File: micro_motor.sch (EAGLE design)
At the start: 56 parts

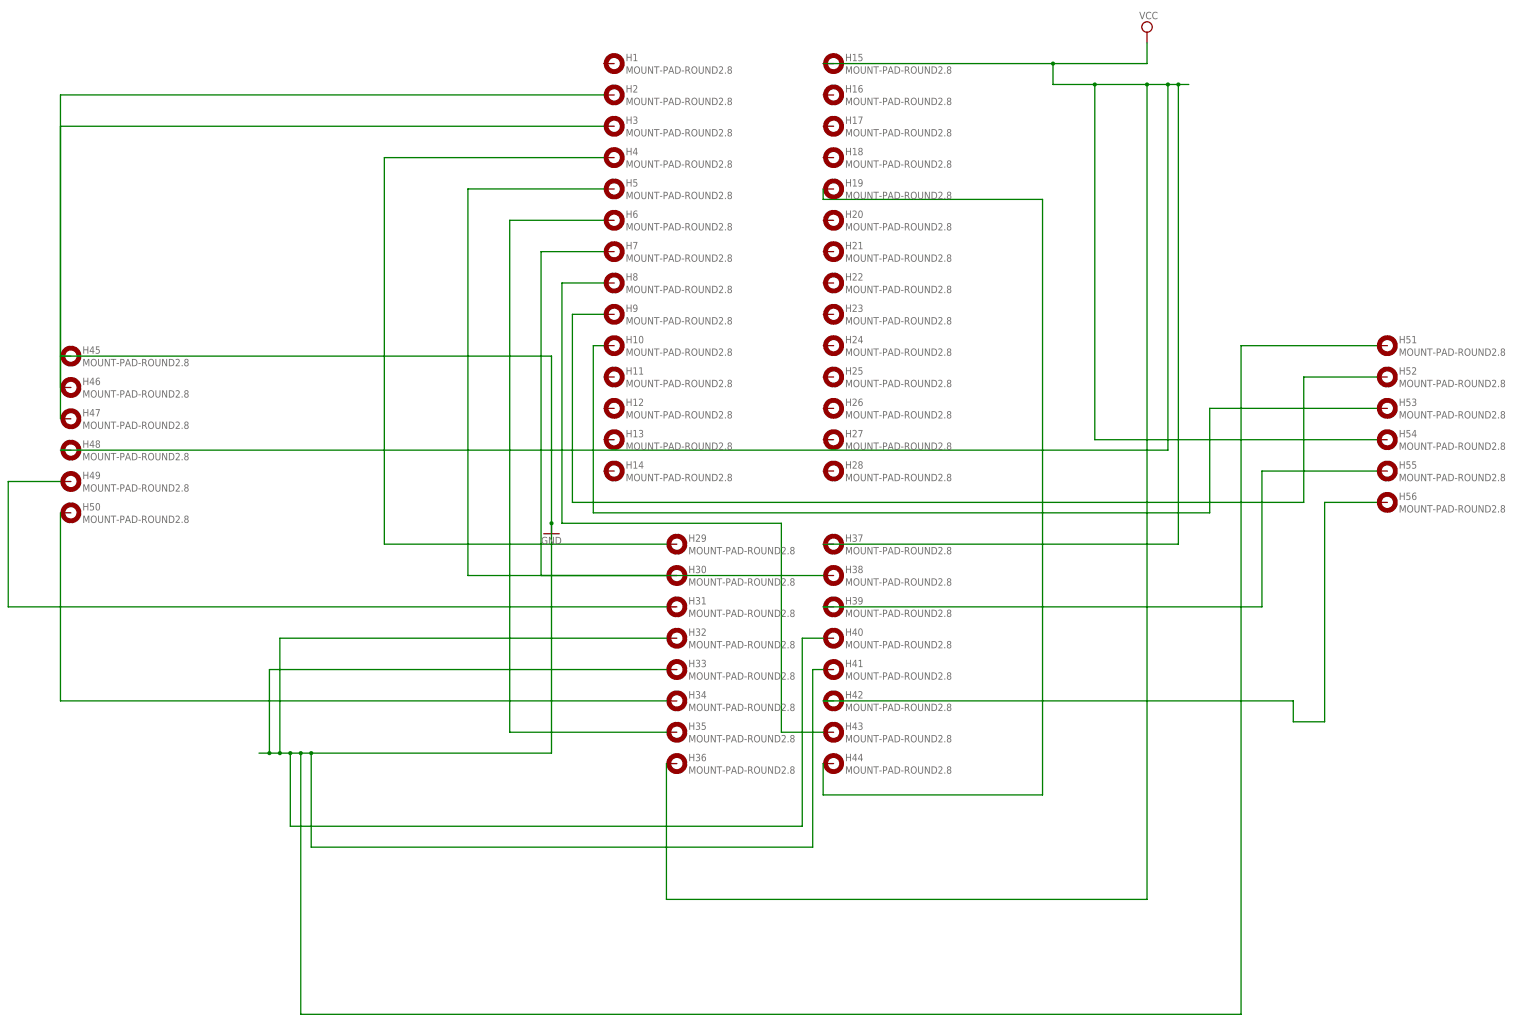
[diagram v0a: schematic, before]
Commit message: Add files via upload
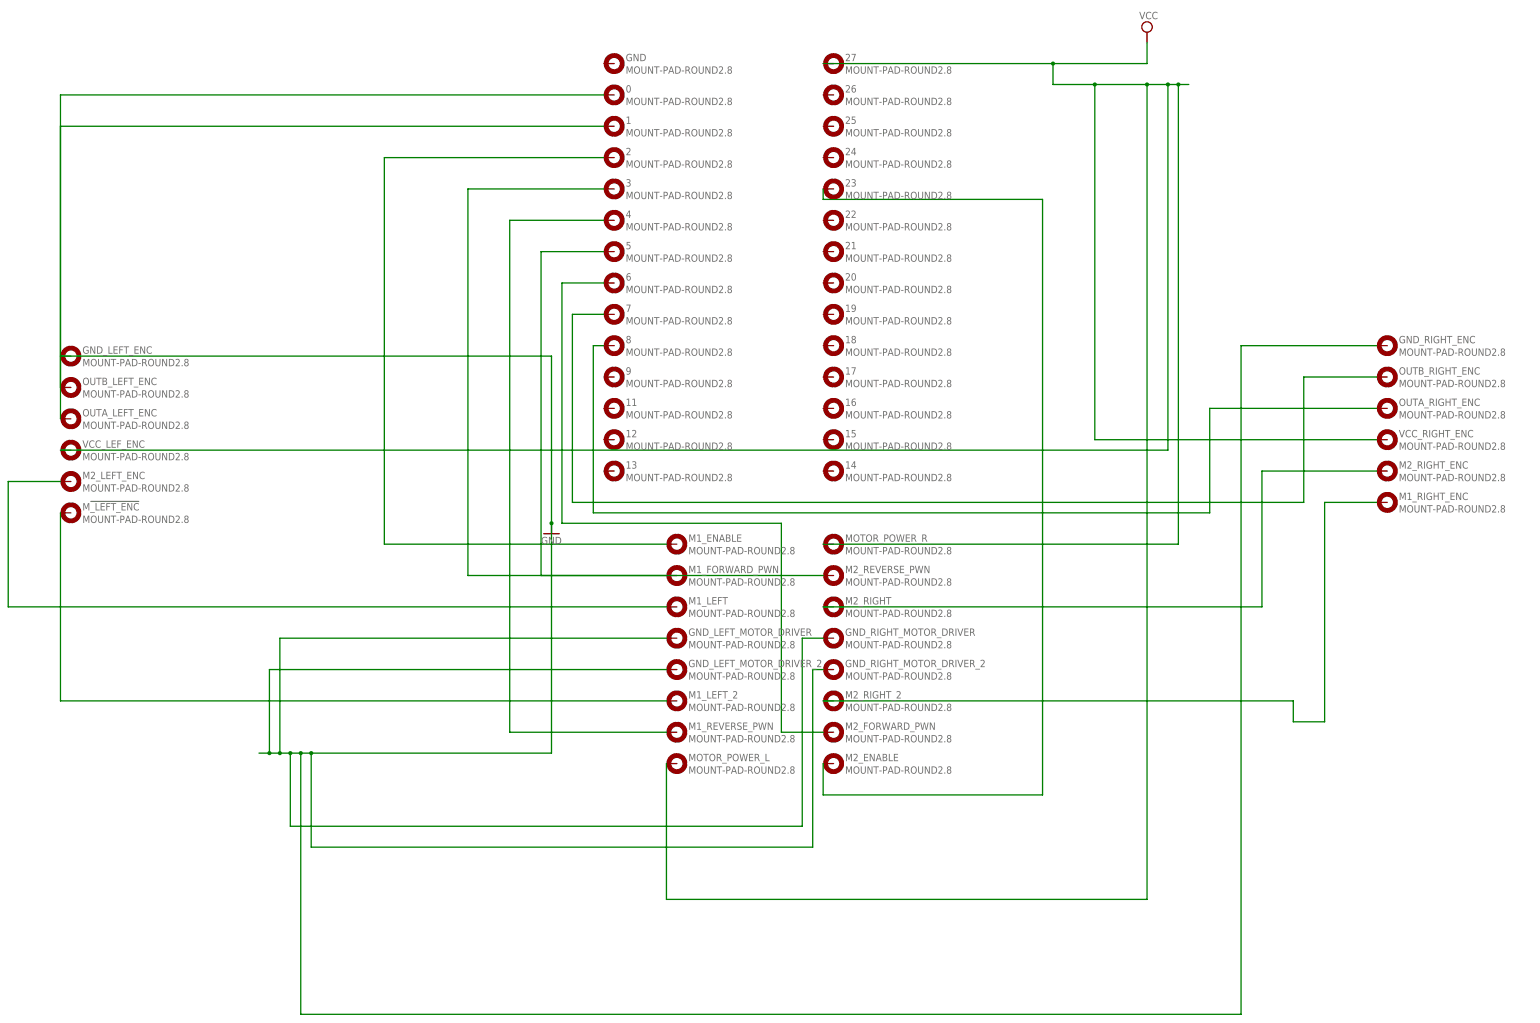
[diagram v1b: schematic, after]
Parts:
- renumbered H1 to GND, H10 to 8, H11 to 9, H12 to 11, H13 to 12, H14 to 13, H15 to 27, H16 to 26, H17 to 25, H18 to 24, H19 to 23, H2 to 0, H20 to 22, H21 to 21, H22 to 20, H23 to 19, H24 to 18, H25 to 17, H26 to 16, H27 to 15, H28 to 14, H29 to M1_ENABLE, H3 to 1, H30 to M1_FORWARD_PWN, H31 to M1_LEFT, H32 to GND_LEFT_MOTOR_DRIVER, H33 to GND_LEFT_MOTOR_DRIVER_2, H34 to M1_LEFT_2, H35 to M1_REVERSE_PWN, H36 to MOTOR_POWER_L, H37 to MOTOR_POWER_R, H38 to M2_REVERSE_PWN, H39 to M2_RIGHT, H4 to 2, H40 to GND_RIGHT_MOTOR_DRIVER, H41 to GND_RIGHT_MOTOR_DRIVER_2, H42 to M2_RIGHT_2, H43 to M2_FORWARD_PWN, H44 to M2_ENABLE, H45 to GND_LEFT_ENC, H46 to OUTB_LEFT_ENC, H47 to OUTA_LEFT_ENC, H48 to VCC_LEF_ENC, H49 to M2_LEFT_ENC, H5 to 3, H50 to M!_LEFT_ENC, H51 to GND_RIGHT_ENC, H52 to OUTB_RIGHT_ENC, H53 to OUTA_RIGHT_ENC, H54 to VCC_RIGHT_ENC, H55 to M2_RIGHT_ENC, H56 to M1_RIGHT_ENC, H6 to 4, H7 to 5, H8 to 6, H9 to 7

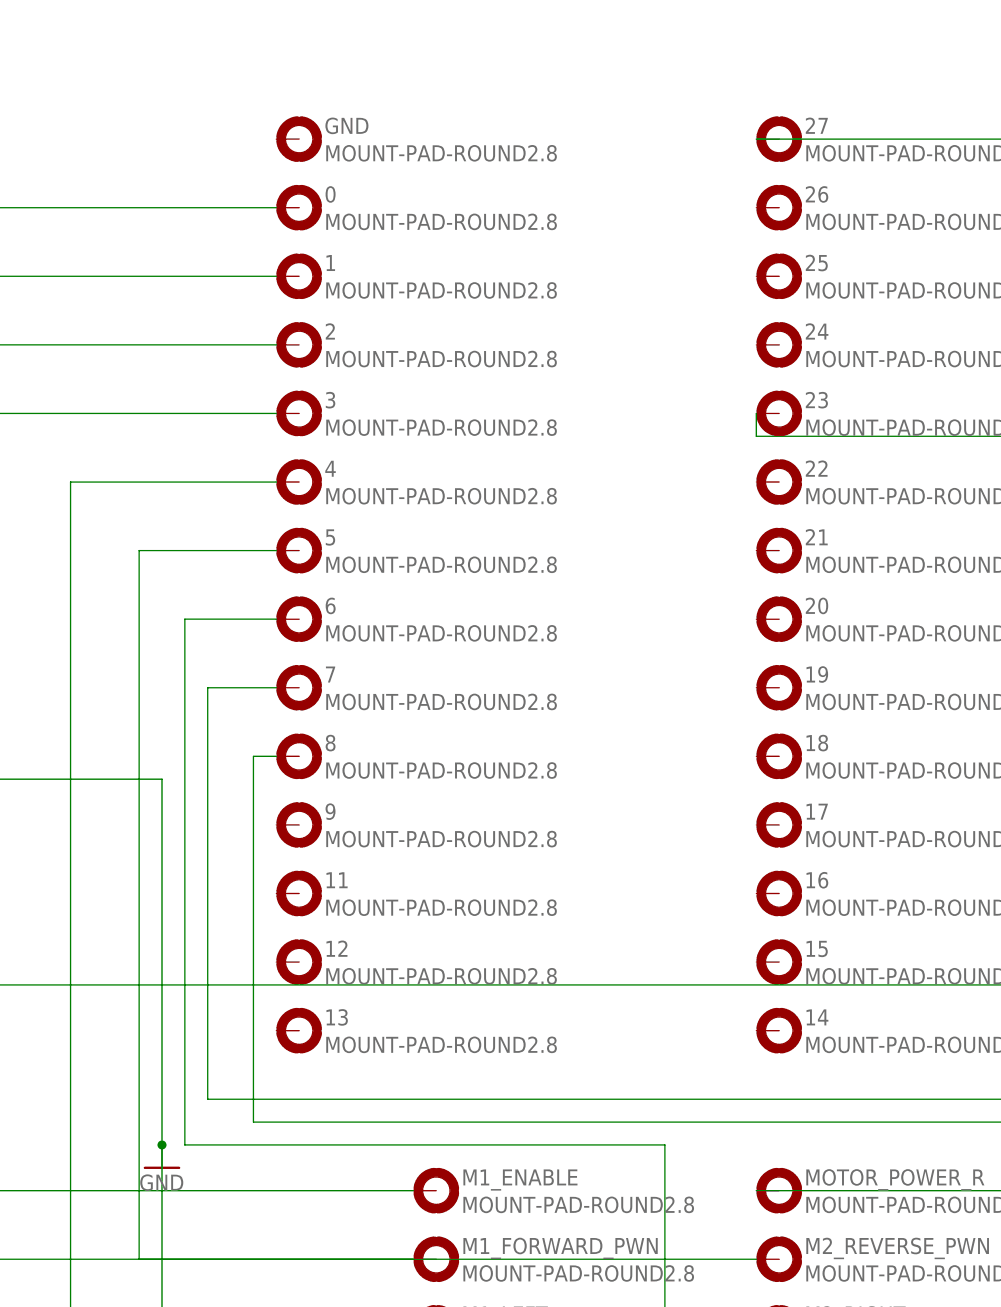
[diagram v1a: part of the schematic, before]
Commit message: Add files via upload
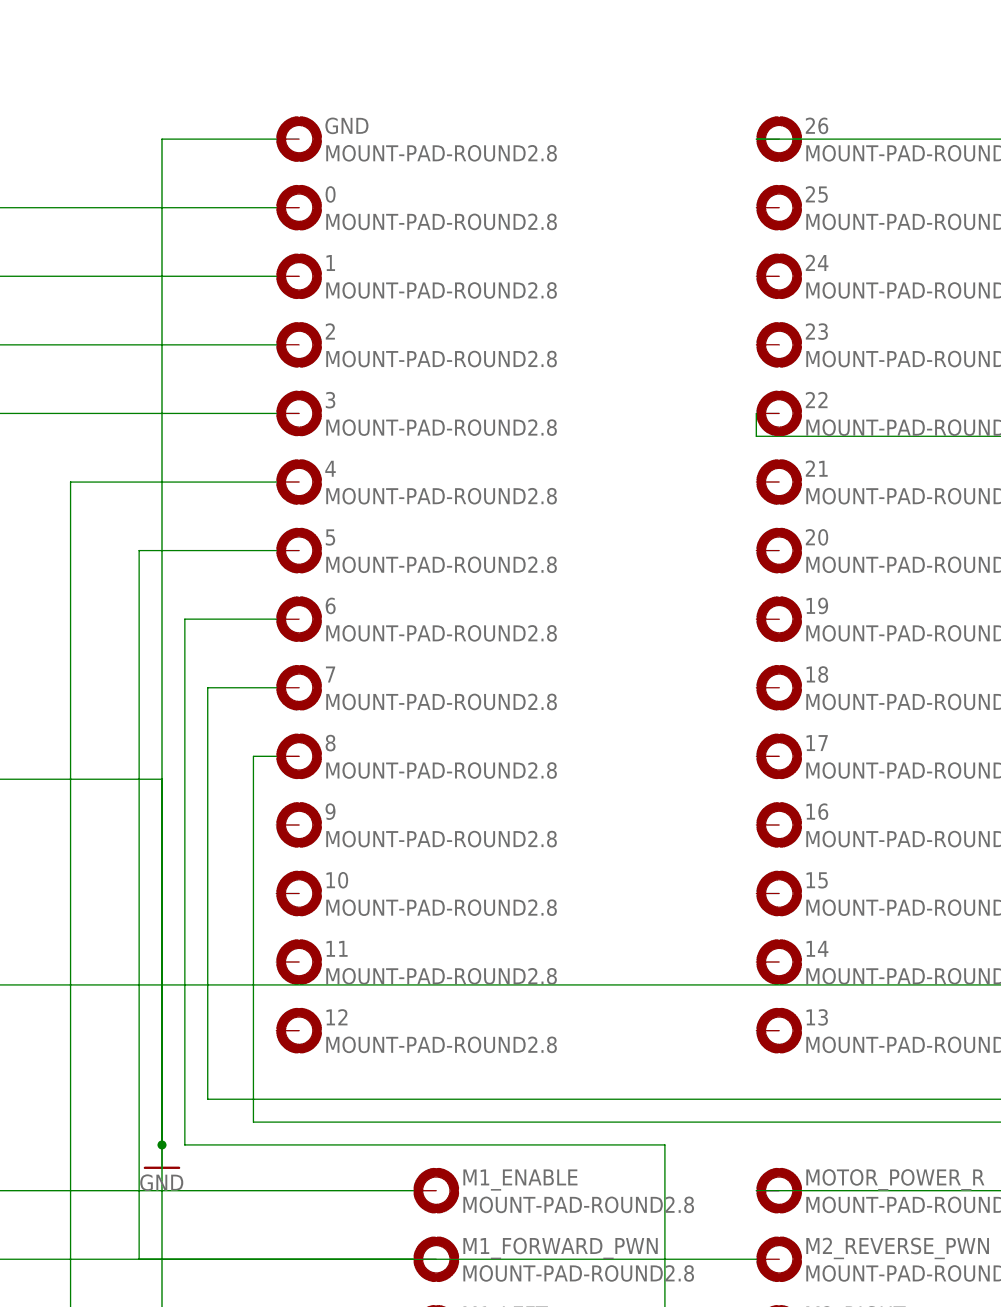
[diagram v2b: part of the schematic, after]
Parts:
- removed 27: MOUNT-PAD-ROUND2.8, holes:MOUNT-PAD-ROUND2.8
- added 10: MOUNT-PAD-ROUND2.8, holes:MOUNT-PAD-ROUND2.8
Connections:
- net GND: now also GND.MOUNT
- net N$13: now also 22.MOUNT; no longer 23.MOUNT
- net VCC: now also 26.MOUNT; no longer 27.MOUNT
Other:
- moved on the sheet: 11, 12, 13, 14, 15, 16, 17, 18, 19, 20, 21, 22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
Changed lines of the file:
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@@
 <part name="8" library="holes" library_urn="urn:adsk.eagle:library:237" deviceset="MOUNT-PAD-ROUND" device="2.8" package3d_urn="urn:adsk.eagle:package:14281/1"/>
 <part name="9" library="holes" library_urn="urn:adsk.eagle:library:237" deviceset="MOUNT-PAD-ROUND" device="2.8" package3d_urn="urn:adsk.eagle:package:14281/1"/>
+<part name="10" library="holes" library_urn="urn:adsk.eagle:library:237" deviceset="MOUNT-PAD-ROUND" device="2.8" package3d_urn="urn:adsk.eagle:package:14281/1"/>
 <part name="11" library="holes" library_urn="urn:adsk.eagle:library:237" deviceset="MOUNT-PAD-ROUND" device="2.8" package3d_urn="urn:adsk.eagle:package:14281/1"/>
 <part name="12" library="holes" library_urn="urn:adsk.eagle:library:237" deviceset="MOUNT-PAD-ROUND" device="2.8" package3d_urn="urn:adsk.eagle:package:14281/1"/>
-<part name="13" library="holes" library_urn="urn:adsk.eagle:library:237" deviceset="MOUNT-PAD-ROUND" device="2.8" package3d_urn="urn:adsk.eagle:package:14281/1"/>
-<part name="27" library="holes" library_urn="urn:adsk.eagle:library:237" deviceset="MOUNT-PAD-ROUND" device="2.8" package3d_urn="urn:adsk.eagle:package:14281/1"/>
 <part name="26" library="holes" library_urn="urn:adsk.eagle:library:237" deviceset="MOUNT-PAD-ROUND" device="2.8" package3d_urn="urn:adsk.eagle:package:14281/1"/>
 <part name="25" library="holes" library_urn="urn:adsk.eagle:library:237" deviceset="MOUNT-PAD-ROUND" device="2.8" package3d_urn="urn:adsk.eagle:package:14281/1"/>
@@
 <part name="15" library="holes" library_urn="urn:adsk.eagle:library:237" deviceset="MOUNT-PAD-ROUND" device="2.8" package3d_urn="urn:adsk.eagle:package:14281/1"/>
 <part name="14" library="holes" library_urn="urn:adsk.eagle:library:237" deviceset="MOUNT-PAD-ROUND" device="2.8" package3d_urn="urn:adsk.eagle:package:14281/1"/>
+<part name="13" library="holes" library_urn="urn:adsk.eagle:library:237" deviceset="MOUNT-PAD-ROUND" device="2.8" package3d_urn="urn:adsk.eagle:package:14281/1"/>
 <part name="M1_ENABLE" library="holes" library_urn="urn:adsk.eagle:library:237" deviceset="MOUNT-PAD-ROUND" device="2.8" package3d_urn="urn:adsk.eagle:package:14281/1"/>
 <part name="M1_FORWARD_PWN" library="holes" library_urn="urn:adsk.eagle:library:237" deviceset="MOUNT-PAD-ROUND" device="2.8" package3d_urn="urn:adsk.eagle:package:14281/1"/>
@@
 <instance part="8" gate="G$1" x="83.82" y="10.16"/>
 <instance part="9" gate="G$1" x="83.82" y="2.54"/>
-<instance part="11" gate="G$1" x="83.82" y="-5.08"/>
-<instance part="12" gate="G$1" x="83.82" y="-12.7"/>
-<instance part="13" gate="G$1" x="83.82" y="-20.32"/>
-<instance part="27" gate="G$1" x="137.16" y="78.74"/>
-<instance part="26" gate="G$1" x="137.16" y="71.12"/>
-<instance part="25" gate="G$1" x="137.16" y="63.5"/>
-<instance part="24" gate="G$1" x="137.16" y="55.88"/>
-<instance part="23" gate="G$1" x="137.16" y="48.26"/>
-<instance part="22" gate="G$1" x="137.16" y="40.64"/>
-<instance part="21" gate="G$1" x="137.16" y="33.02"/>
-<instance part="20" gate="G$1" x="137.16" y="25.4"/>
-<instance part="19" gate="G$1" x="137.16" y="17.78"/>
-<instance part="18" gate="G$1" x="137.16" y="10.16"/>
-<instance part="17" gate="G$1" x="137.16" y="2.54"/>
-<instance part="16" gate="G$1" x="137.16" y="-5.08"/>
-<instance part="15" gate="G$1" x="137.16" y="-12.7"/>
-<instance part="14" gate="G$1" x="137.16" y="-20.32"/>
+<instance part="10" gate="G$1" x="83.82" y="-5.08"/>
+<instance part="11" gate="G$1" x="83.82" y="-12.7"/>
+<instance part="12" gate="G$1" x="83.82" y="-20.32"/>
+<instance part="26" gate="G$1" x="137.16" y="78.74"/>
+<instance part="25" gate="G$1" x="137.16" y="71.12"/>
+<instance part="24" gate="G$1" x="137.16" y="63.5"/>
+<instance part="23" gate="G$1" x="137.16" y="55.88"/>
+<instance part="22" gate="G$1" x="137.16" y="48.26"/>
+<instance part="21" gate="G$1" x="137.16" y="40.64"/>
+<instance part="20" gate="G$1" x="137.16" y="33.02"/>
+<instance part="19" gate="G$1" x="137.16" y="25.4"/>
+<instance part="18" gate="G$1" x="137.16" y="17.78"/>
+<instance part="17" gate="G$1" x="137.16" y="10.16"/>
+<instance part="16" gate="G$1" x="137.16" y="2.54"/>
+<instance part="15" gate="G$1" x="137.16" y="-5.08"/>
+<instance part="14" gate="G$1" x="137.16" y="-12.7"/>
+<instance part="13" gate="G$1" x="137.16" y="-20.32"/>
 <instance part="M1_ENABLE" gate="G$1" x="99.06" y="-38.1"/>
 <instance part="M1_FORWARD_PWN" gate="G$1" x="99.06" y="-45.72"/>
@@
 <segment>
 <pinref part="SUPPLY1" gate="G$1" pin="VCC"/>
-<pinref part="27" gate="G$1" pin="MOUNT"/>
+<pinref part="26" gate="G$1" pin="MOUNT"/>
 <wire x1="213.36" y1="83.82" x2="213.36" y2="78.74" width="0.1524" layer="91"/>
 <wire x1="213.36" y1="78.74" x2="190.5" y2="78.74" width="0.1524" layer="91"/>
@@
 <wire x1="10.16" y1="-111.76" x2="10.16" y2="-88.9" width="0.1524" layer="91"/>
 <junction x="10.16" y="-88.9"/>
+<pinref part="GND" gate="G$1" pin="MOUNT"/>
+<wire x1="81.28" y1="78.74" x2="68.58" y2="78.74" width="0.1524" layer="91"/>
+<wire x1="68.58" y1="78.74" x2="68.58" y2="-33.02" width="0.1524" layer="91"/>
 </segment>
 </net>
@@
 <wire x1="134.62" y1="-99.06" x2="187.96" y2="-99.06" width="0.1524" layer="91"/>
 <wire x1="187.96" y1="-99.06" x2="187.96" y2="45.72" width="0.1524" layer="91"/>
-<pinref part="23" gate="G$1" pin="MOUNT"/>
+<pinref part="22" gate="G$1" pin="MOUNT"/>
 <wire x1="187.96" y1="45.72" x2="134.62" y2="45.72" width="0.1524" layer="91"/>
 <wire x1="134.62" y1="45.72" x2="134.62" y2="48.26" width="0.1524" layer="91"/>
